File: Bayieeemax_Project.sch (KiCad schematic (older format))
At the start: 35 parts, among them J1 Baterry_P.IN, J10 MicroStep_1/32, J11 Motor1, J12 Motor2, J13 Motor3, J14 Motor4, J15 Motor5, J16 Motor6, J2 USB_TTL, J3 Raspberry_POWER_IN, J4 ACS_SENSOR, J5 I2C_MPU_Raspberry, J6 GPS_Conn, J7 TTL_Raspberry, J8 I2C_MAX30100_Raspberry, J9 MicroStep_1/16, U1 MPU-9250, U2 ChinaBluePill, U3 MAX30100EFD+

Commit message: New files
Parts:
- removed U3: MAX30100EFD+, LGA14R80P2X7_560X280X130, symbol Bayieeemax_Project-rescue:MAX30100EFD+
- added C8: 100nf, Capacitor_SMD:C_Elec_6.3x7.7, symbol Device:C
- added J17: i2C_MAX30100, Connector_PinSocket_2.54mm:PinSocket_1x06_P2.54mm_Vertical, symbol Connector_Generic:Conn_01x07
- added R3, R4: 10K, Resistor_THT:R_Axial_DIN0207_L6.3mm_D2.5mm_P10.16mm_Horizontal, symbol Device:R
- C1: footprint (none) -> Capacitor_THT:C_Radial_D10.0mm_H12.5mm_P5.00mm
- C2, C3, C4, C5, C6, C7: footprint (none) -> Capacitor_SMD:C_Elec_6.3x7.7
- J1, J3: footprint (none) -> Baiyeeemax:TerminalBlock_Phoenix_PT-1,5-2-5.0-H_1x02_P5.00mm_Horizontal
- J10, J9: footprint (none) -> Connector_PinHeader_2.00mm:PinHeader_2x03_P2.00mm_Vertical
- J11, J12, J13, J14, J15, J16: footprint (none) -> Connector_PinHeader_2.00mm:PinHeader_1x04_P2.00mm_Vertical
- J2: footprint (none) -> Connector_PinHeader_2.54mm:PinHeader_1x06_P2.54mm_Vertical
- J4: footprint (none) -> Connector_PinHeader_2.54mm:PinHeader_1x03_P2.54mm_Vertical
- J5, J7, J8: footprint (none) -> Connector_PinHeader_2.54mm:PinHeader_1x02_P2.54mm_Vertical
- J6: footprint (none) -> Connector_Molex:Molex_MicroClasp_55935-0630_1x06_P2.00mm_Horizontal
- R1, R2: footprint (none) -> Resistor_THT:R_Axial_DIN0207_L6.3mm_D2.5mm_P10.16mm_Horizontal
- U1: footprint QFN40P300X300X105-24N -> Baiyeeemax:QFN40P300X300X105-24N
- U2: footprint (none) -> Baiyeeemax:BluePill_STM32F103C
- VR1: footprint CONV_XL4015 -> Baiyeeemax:DCDC_stepdown_75W-XL4015
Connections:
- net labels added: ~INT_MAX3100
- net labels removed: +3V0, EN_GPS, GND_GPS, PPS_GPS, VCC3V3_GPS
- wire segments 232 -> 254
- no-connect marks 35 -> 47
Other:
- note added: "En"
- note added: "GND\n"
- note added: "Microcontroller\n"
- note added: "Power_source\n"
- note added: "Sensors\n"
- note added: "Step Motor + Drivers + Step Mode\n"
- note added: "VCC3.3V\n"
- note removed: "5V pwm tolerant\n"
- moved on the sheet: J2, J3, J4, J5, J7, J8, R1, R2, U1, U2, VR1

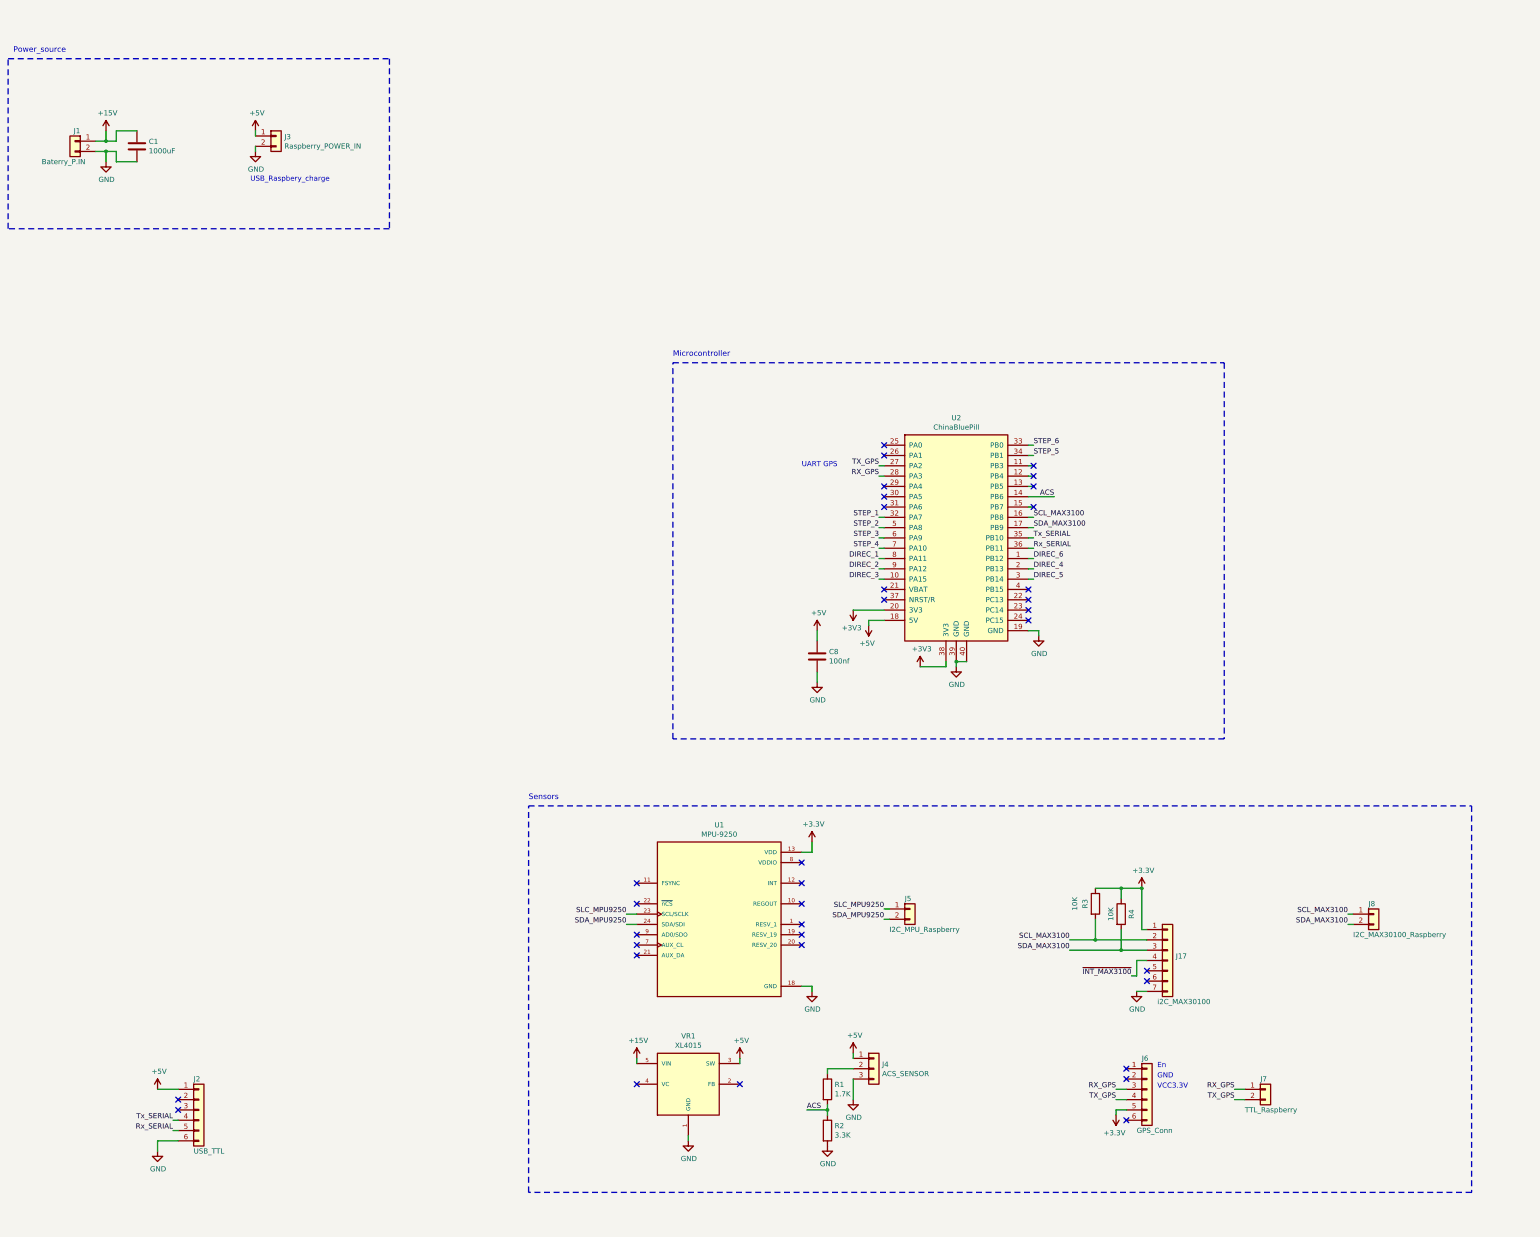
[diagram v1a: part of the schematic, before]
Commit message: Changes
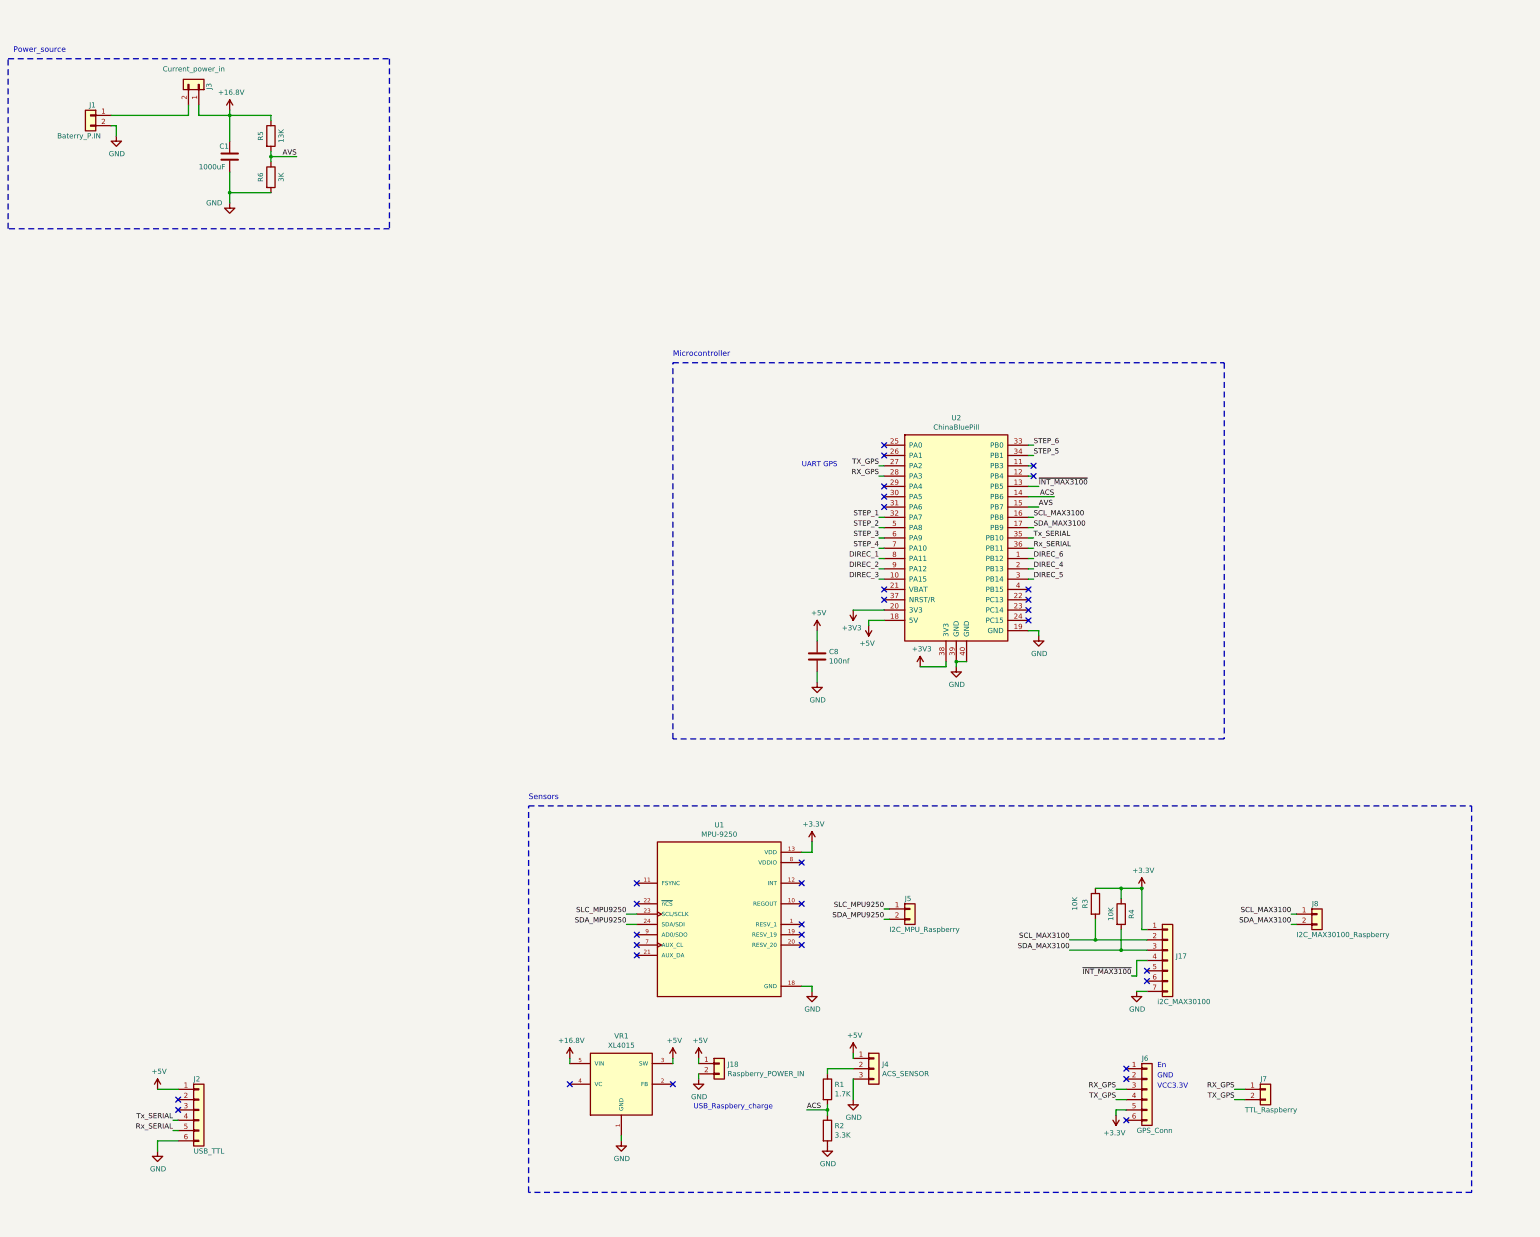
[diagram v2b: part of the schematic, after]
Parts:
- added J18: Raspberry_POWER_IN, Baiyeeemax:TerminalBlock_Phoenix_PT-1,5-2-5.0-H_1x02_P5.00mm_Horizontal, symbol Connector_Generic:Conn_01x02
- added R5: 13K, Resistor_THT:R_Axial_DIN0207_L6.3mm_D2.5mm_P10.16mm_Horizontal, symbol Device:R
- added R6: 3K, Resistor_THT:R_Axial_DIN0207_L6.3mm_D2.5mm_P10.16mm_Horizontal, symbol Device:R
- J3: value Raspberry_POWER_IN -> Current_power_in
- U1: footprint Baiyeeemax:QFN40P300X300X105-24N -> Baiyeeemax:MPU-9250
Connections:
- net +15V: no longer C1.2, J1.1 (Pin_1), VR1.5 (VIN)
- net +5V: now also J18.1 (Pin_1); no longer J3.1 (Pin_1)
- net GND: now also J18.2 (Pin_2), R6.2; no longer J3.2 (Pin_2)
- net ~INT_MAX3100: now also U2.13 (PB5)
- net AVS: now reaches U2.15 (PB7)
- net AVS: now also R5.2, R6.1
- new net: J1.1 (Pin_1), J3.2 (Pin_2)
- new net +12V: C1.2, J3.1 (Pin_1), R5.1, VR1.5 (VIN)
- no-connect marks 47 -> 45
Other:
- moved on the sheet: C1, J1, J8, VR1
